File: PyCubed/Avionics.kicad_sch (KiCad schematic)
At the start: 49 parts, among them IC3 UA741IDT, J19 F3311A7H121014E200, J8 Conn_01x09, U1 MAX706RESA, U2 ATSAMD51J19A-AU, U3 BMX160, Y1 32.768kHz

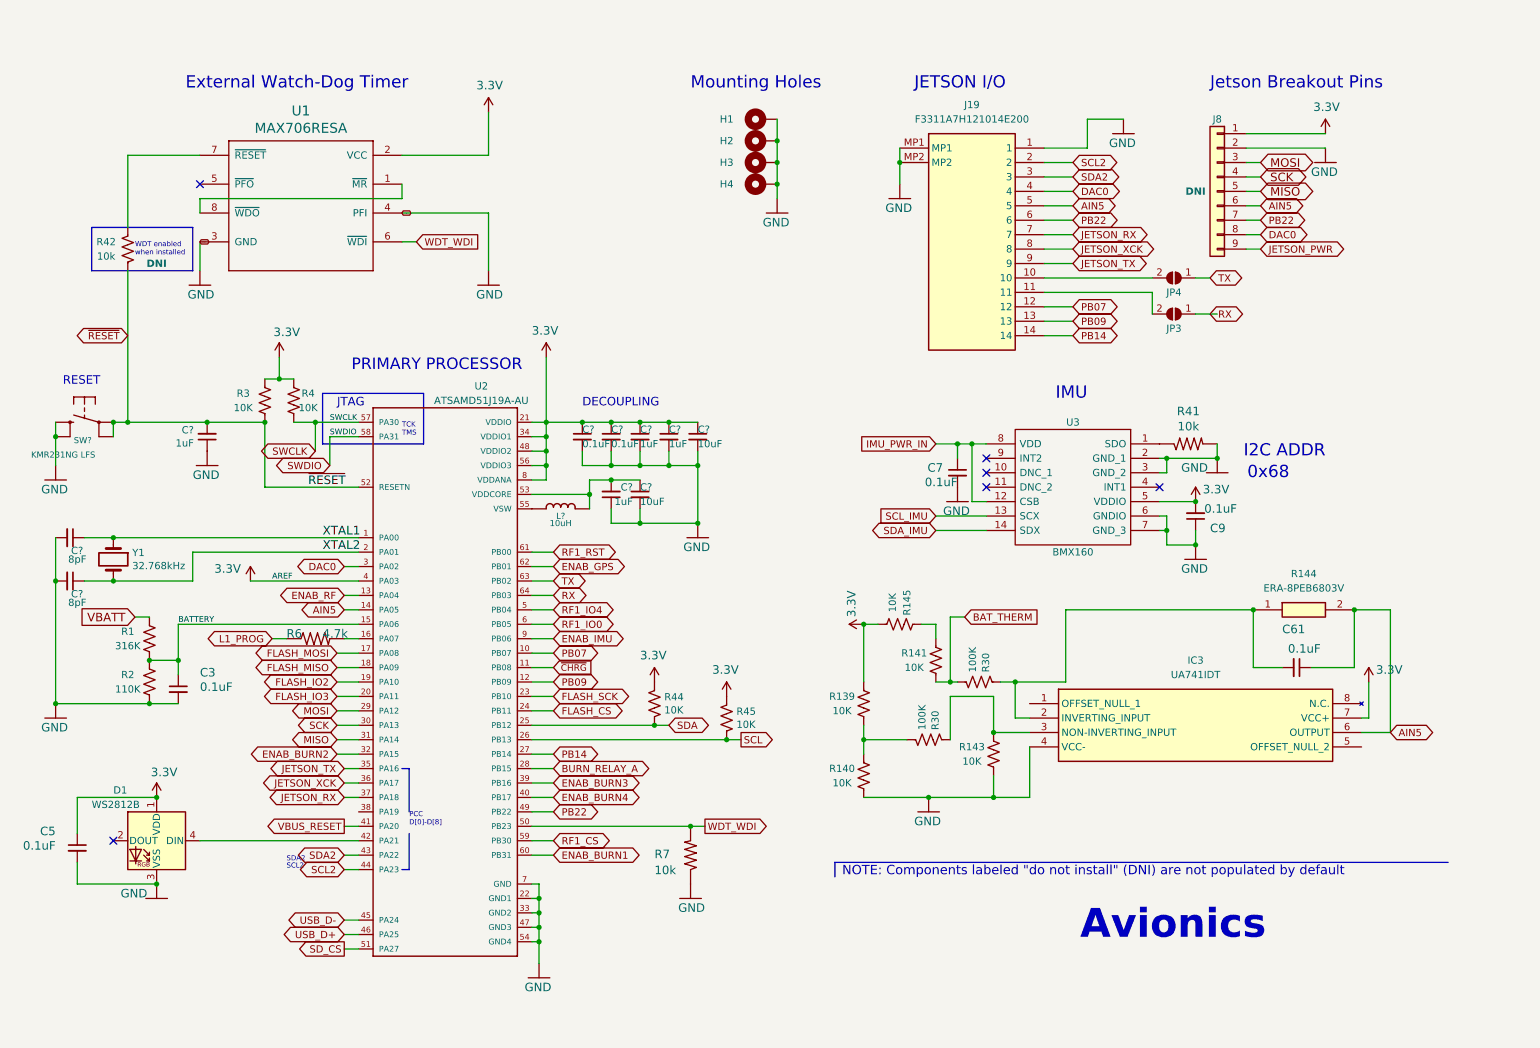
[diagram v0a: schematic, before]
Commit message: PyCubed Routing Done
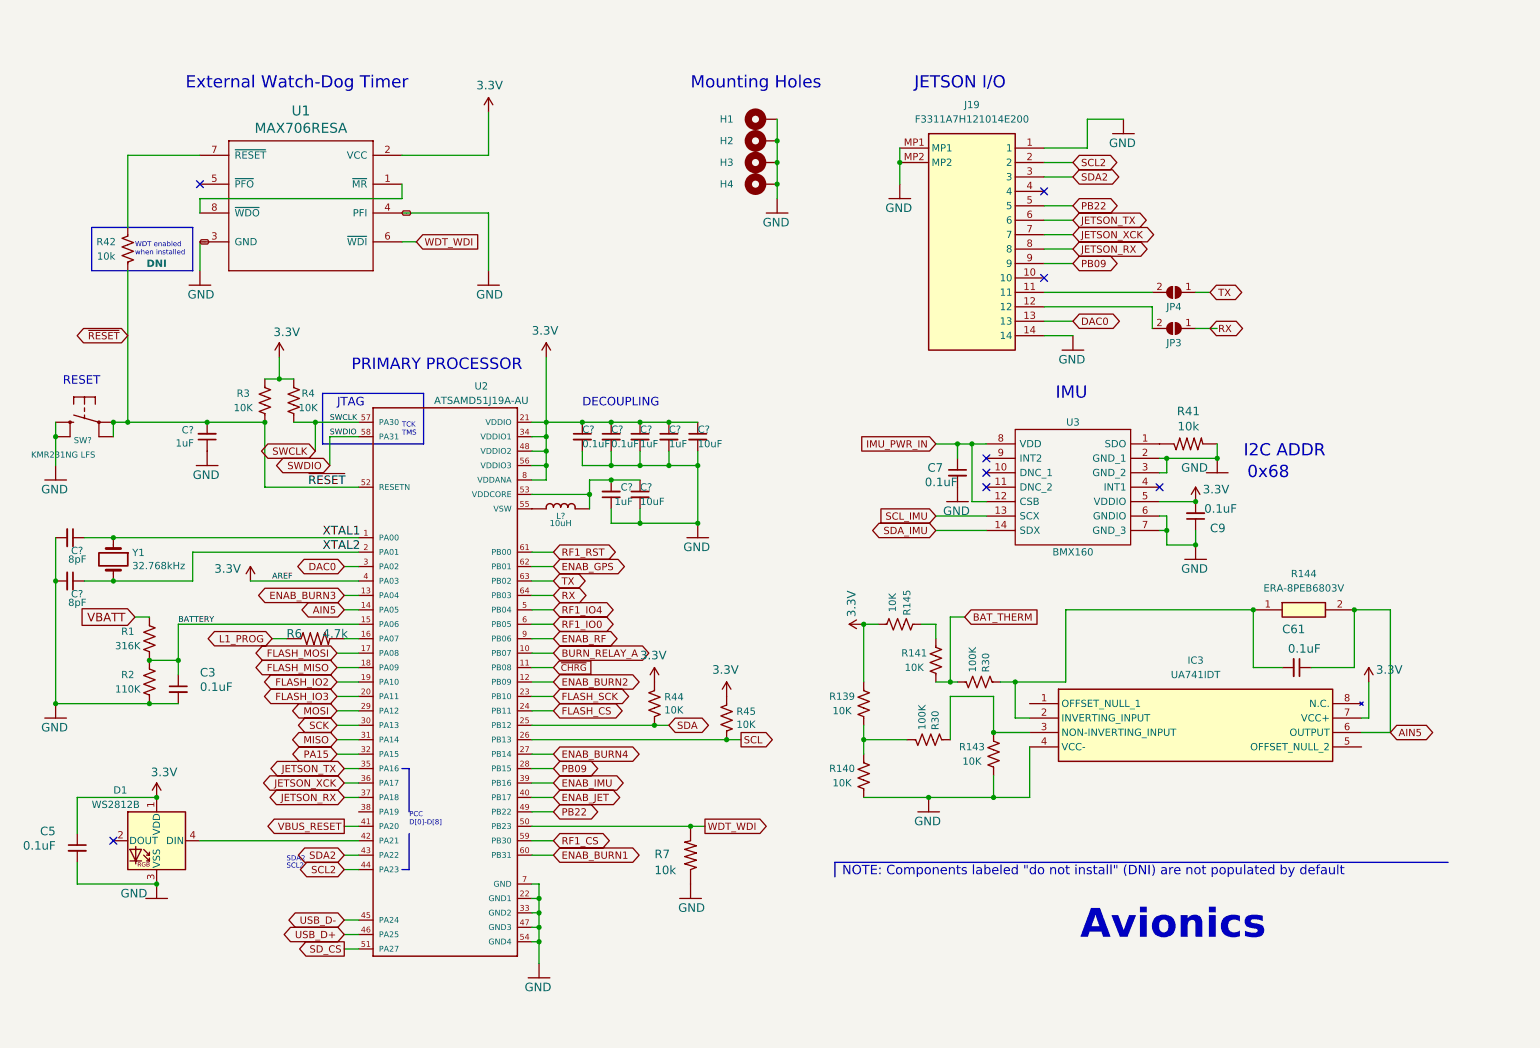
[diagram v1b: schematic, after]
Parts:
- removed J8: Conn_01x09, Connector_PinHeader_2.54mm:PinHeader_1x09_P2.54mm_Vertical, symbol Connector_Generic:Conn_01x09
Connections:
- net AIN5: no longer J19.5
- net BURN_RELAY_A: now also U2.10 (PB07); no longer U2.28 (PB15)
- net DAC0: now also J19.13; no longer J19.4
- net ENAB_BURN2: now also U2.12 (PB09); no longer U2.32 (PA15)
- net ENAB_BURN3: now also U2.13 (PA04); no longer U2.39 (PB16)
- net ENAB_BURN4: now also U2.27 (PB14); no longer U2.40 (PB17)
- net ENAB_IMU: now also U2.39 (PB16); no longer U2.9 (PB06)
- net ENAB_RF: now also U2.9 (PB06); no longer U2.13 (PA04)
- net GND: now also J19.14
- net JETSON_RX: now also J19.8; no longer J19.7
- net JETSON_TX: now also J19.6; no longer J19.9
- net JETSON_XCK: now also J19.7; no longer J19.8
- net PB09: now also J19.9, U2.28 (PB15); no longer J19.13, U2.12 (PB09)
- net PB22: now also J19.5; no longer J19.6
- net at JP4.2 (B): now also J19.11; no longer J19.10
- net at JP3.2 (B): now also J19.12; no longer J19.11
- removed net PB07: J19.12, U2.10 (PB07)
- removed net PB14: J19.14, U2.27 (PB14)
- new net ENAB_JET: U2.40 (PB17)
- new net PA15: U2.32 (PA15)
- no-connect marks 6 -> 8
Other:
- note removed: "Jetson Breakout Pins"

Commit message: Mainboard Final Design
Updated BMS
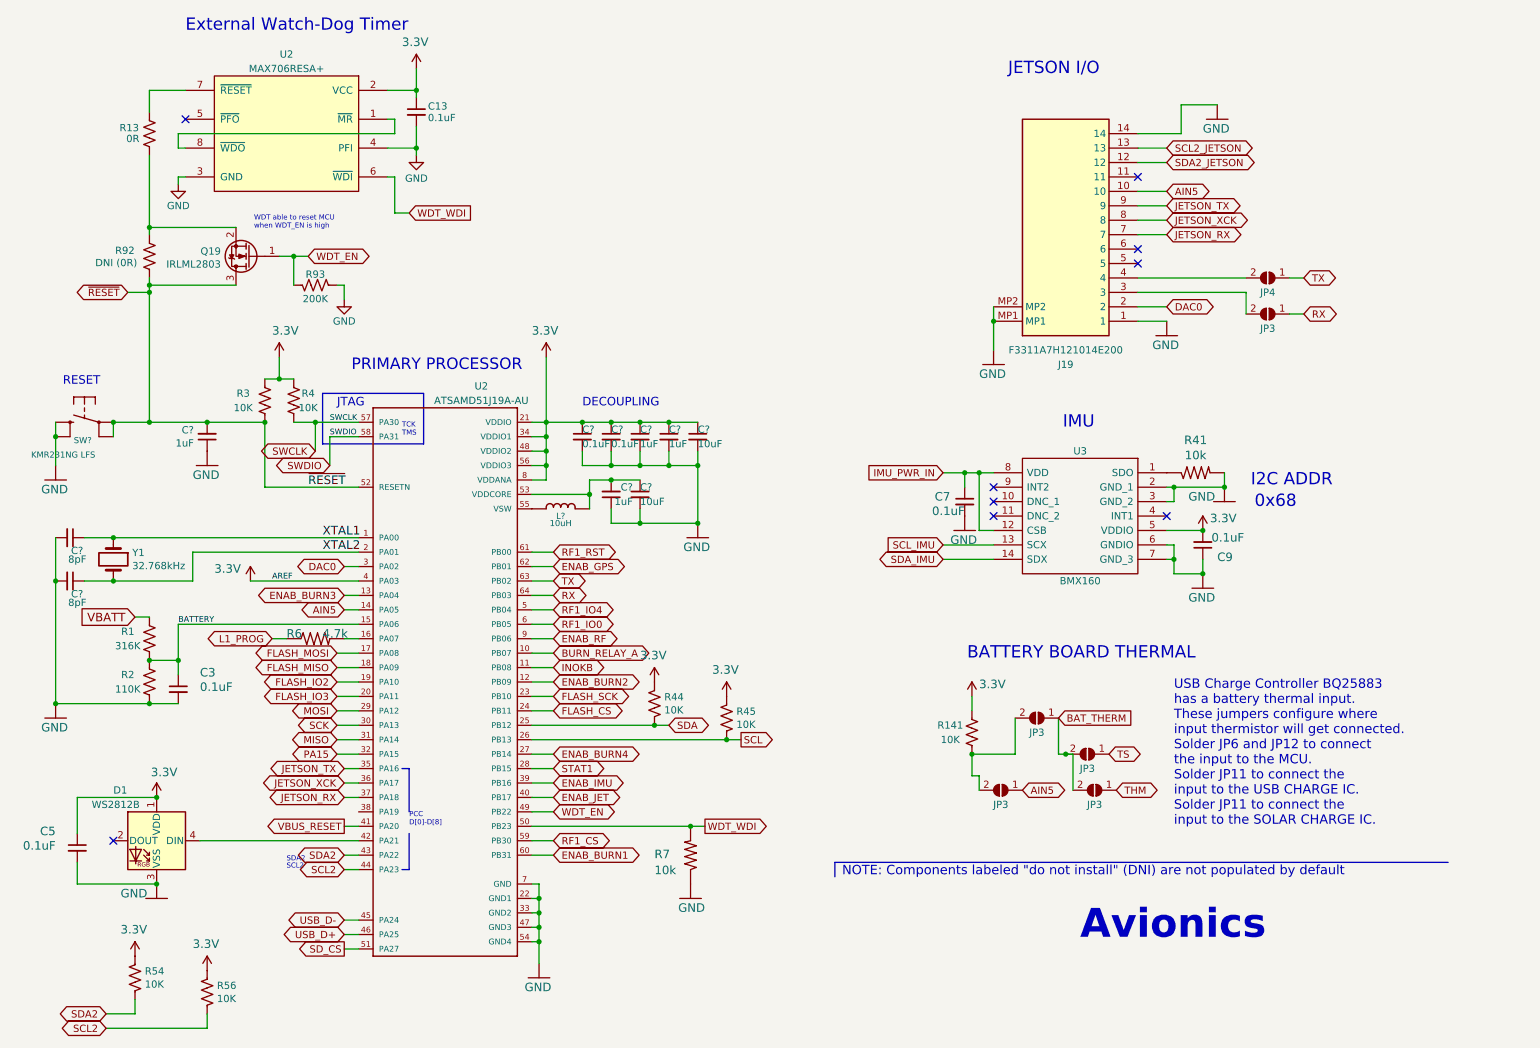
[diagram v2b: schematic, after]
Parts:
- removed C61: 0.1uF, Capacitor_SMD:C_0603_1608Metric, symbol mainboard:C_Small
- removed H1, H2, H3, H4: MountingHole_Pad, MountingHole:MountingHole_3.2mm_M3_DIN965_Pad, symbol Mechanical:MountingHole_Pad
- removed IC3: UA741IDT, SOIC127P600X175-8N, symbol SamacSys_Parts:UA741IDT
- removed R139, R140, R143, R145: 10K, Resistor_SMD:R_0603_1608Metric, symbol Device:R_US
- removed R144: ERA-8PEB6803V, ERA8P, symbol SamacSys_Parts:ERA-8PEB6803V
- removed R30 (x2): 100K, Resistor_SMD:R_0603_1608Metric, symbol Device:R_US
- removed R42: 10k, Resistor_SMD:R_0603_1608Metric, symbol Device:R_US
- removed U1: MAX706RESA, Package_SO:SO-8_3.9x4.9mm_P1.27mm, symbol mainboard:MAX708RESA-T
- added C13: 0.1uF, Capacitor_SMD:C_0603_1608Metric, symbol Device:C_Small
- added JP3 (x4): SolderJumper_2_Open, Jumper:SolderJumper-2_P1.3mm_Open_Pad1.0x1.5mm, symbol Jumper:SolderJumper_2_Open
- added Q19: IRLML2803, Package_TO_SOT_SMD:SOT-23, symbol Transistor_FET:IRLML2060
- added R13: 0R, Resistor_SMD:R_0603_1608Metric, symbol Device:R_US
- added R54, R56: 10K, Resistor_SMD:R_0603_1608Metric, symbol Device:R_US
- added R92: DNI (0R), Resistor_SMD:R_0603_1608Metric, symbol Device:R_US
- added R93: 200K, Resistor_SMD:R_0603_1608Metric, symbol Device:R_US
- added U2: MAX706RESA+, Package_SO:SOIC-8_3.9x4.9mm_P1.27mm, symbol mainboard:MAX708RESA+
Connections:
- net 3.3V: now also R141.1, C13.1, R54.1, R56.1, U2.2 (VCC)
- net AIN5: now also J19.10, JP3.1 (A)
- net BAT_THERM: now also JP3.1 (A), JP3.2 (B), JP3.2 (B); no longer R141.2
- net DAC0: now also J19.2; no longer J19.13
- net GND: now also C13.2, R93.2, U2.3 (GND), U2.4 (PFI)
- net JETSON_RX: now also J19.7; no longer J19.8
- net JETSON_TX: now also J19.9; no longer J19.6
- net JETSON_XCK: now also J19.8; no longer J19.7
- net SCL2: now also R56.2; no longer J19.2
- net SDA2: now also R54.2; no longer J19.3
- net WDT_WDI: now also U2.6 (~{WDI})
- net ~{RESET}: now also Q19.3 (D), R92.1
- net at JP3.2 (B): now also J19.3; no longer J19.12
- net at JP4.2 (B): now also J19.4; no longer J19.11
- net PB09 renamed STAT1
- net STAT1: no longer J19.9
- net PB22: no longer names the net of J19.5
- net PB22: no longer U2.49 (PB22)
- net ~{CHRG} renamed INOKB
- new net: JP3.2 (B), JP3.2 (B), R141.2
- new net: U2.1 (~{MR}), U2.8 (~{WDO})
- new net: R13.2, U2.7 (~{RESET})
- new net: Q19.2 (S), R13.1, R92.2
- new net SCL2_JETSON: J19.13
- new net SDA2_JETSON: J19.12
- new net THM: JP3.1 (A)
- new net TS: JP3.1 (A)
- new net WDT_EN: Q19.1 (G), R93.1, U2.49 (PB22)
- no-connect marks 8 -> 9
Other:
- note added: "BATTERY BOARD THERMAL"
- note added: "USB Charge Controller BQ25883 has a battery thermal input. These jumpers configure where input thermistor will get connected. Solder JP6 and JP12 to connect the input to the MCU. Solder JP11 to connect the input to the USB CHARGE IC. Solder JP11 to connect the input to the SOLAR CHARGE IC."
- note added: "WDT able to reset MCU when WDT_EN is high"
- note removed: "Mounting Holes"
- note removed: "WDT enabled when installed"
- moved on the sheet: C7, C9, J19, JP3, JP4, R141, R41, U3
